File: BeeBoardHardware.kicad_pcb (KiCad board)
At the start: 4 copper layers, 29.4 x 34.1 mm, 44 parts, among them J2 USB_C_Receptacle_USB2.0_16P, J3 Conn_01x02, J4 Conn_01x11, Q1 AO3413, SW2 SW_Push, U1 MCP16311T-E/MNY, U2 BQ24074RGTT, U3 USBLC6-2SC6, U4 LC709203FQH-01TWG, U5 STM6600DQ25DM6F

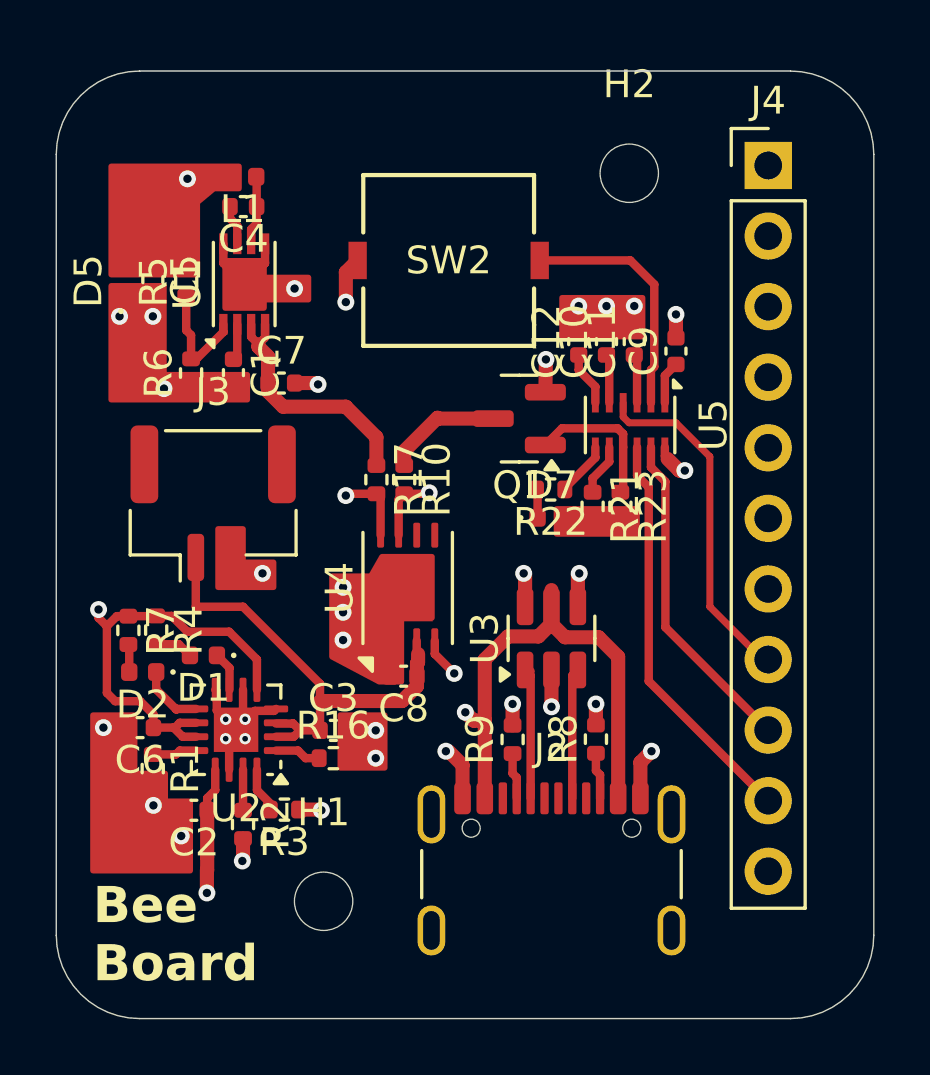
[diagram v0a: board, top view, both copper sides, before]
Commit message: finish routes
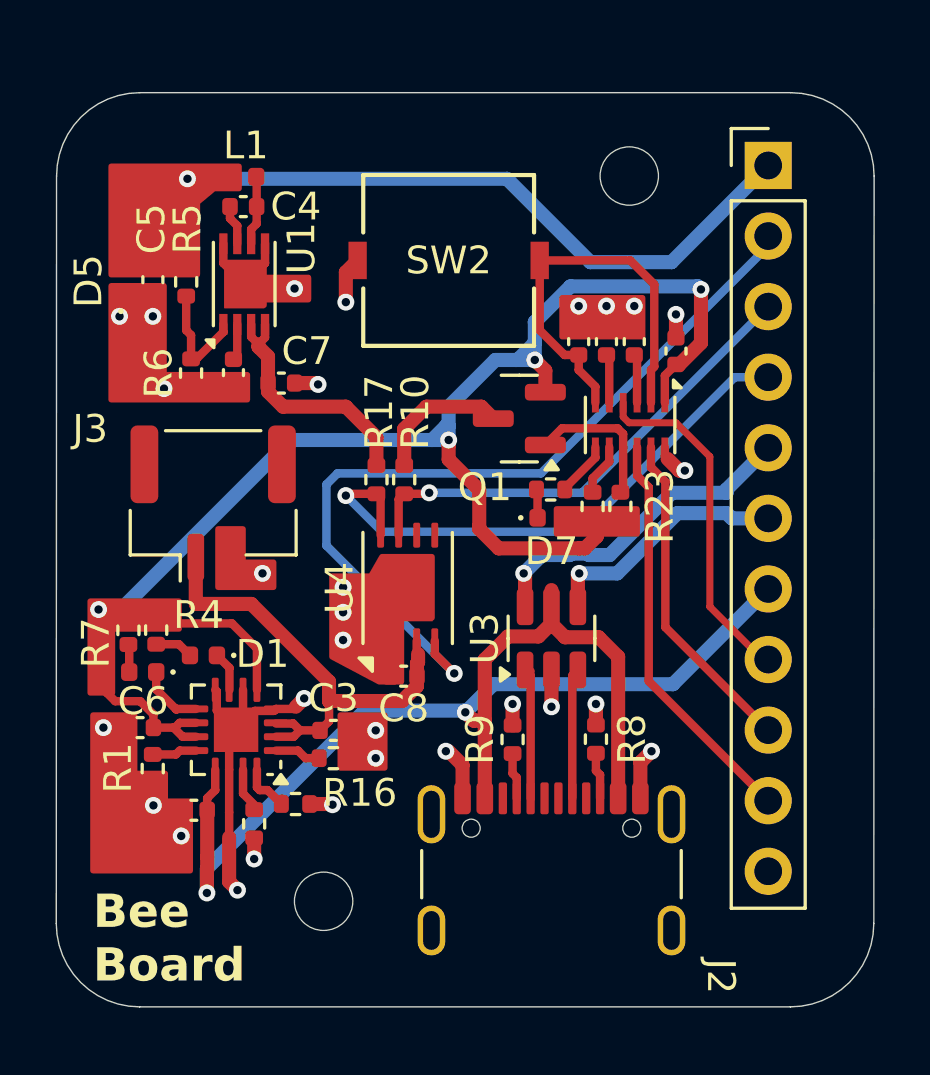
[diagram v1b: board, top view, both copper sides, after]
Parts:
- moved R3 0.45 mm to (79.8, 87.3)
- moved R2 0.40 mm to (78.3, 88.0)
- moved H2 0.10 mm to (91.8, 64.7)
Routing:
- net PWR PTH: track 20.3 -> 62.6 mm, vias 2 -> 4
- net BAT_ALERT: track 1.61 -> 30.1 mm
- net VBUS: track 23.1 -> 48.4 mm
- net +3v3: track 7.14 -> 30.7 mm
- net BAT_SCL: track 2.68 -> 20.7 mm
- net BAT_SDA: track 2.57 -> 17.5 mm
- net USB_D-: track 1.22 -> 12.0 mm
- net USB_D+: track 1.22 -> 9.00 mm
- net GND: track 33.2 -> 38.2 mm, vias 31 -> 29
- net Net-(U5-~{PB}): track 10.8 -> 15.0 mm
- net PWR: track 13.3 -> 14.1 mm
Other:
- board size 29.4 x 34.1 mm -> 29.4 x 32.9 mm
